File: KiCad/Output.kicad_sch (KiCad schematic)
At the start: 644 parts, among them J1 R_Phono_In, J10 VCC_IN, J11 VCC_OUT, J12 EMK_In, J15 Mic_Effekt_Out, J16 Mic_Effekt_Out, J17 Mic_Effekt_Out, J18 Mic_Effekt_Out, J19 Phono/Line_Out, J2 L_Phono_In, J20 Mic_Effekt_Out, J21 Conn_01x05_bridged, J22 EMK_In, J24 Mic_Effekt_In, J25 Mic_Effekt_In, J26 Phono/Line_In, J27 Mic_Effekt_In, J28 Pegel_Out, J29 Pegel_Out, J3 R_Line_In, J30 Pegel_In, J31 Pegel_In, J32 Pegel_In, J33 Pegel_In, J34 LED_Out, J35 LED_In, J36 VU_Meter_Out, J37 AUX_Send_3, J38 AUX_Send_1, J39 AUX_Send_2, J4 L_Line_In, J40 Bass_Out, J41 Kick_Out, J42 Mid_Out, J43 High_Out, J44 Line_Out_L, J45 Line_Out_R, J5 Mic_In, J6 Effekt_In, J7 AUX_RET_1, J8 AUX_RET_2, J9 AUX_RET_3, SW1 SW_DPST, SW10 SW_SPDT, SW11 SW_SPDT, SW12 SW_SPDT, SW2 SW_SPDT, SW3 SW_SPDT, SW4 SW_SPDT, SW5 SW_SPDT, SW6 SW_SPDT, SW7 SW_SPDT, SW8 SW_SPDT, SW9 SW_Rotary_1x4, U1 TL074, U10 TL074, U11 TL074, U12 TL074, U13 TL074, U14 TL074, U15 TL074, U16 TL074, U17 TL074, U18 TL074, U19 TL074, U2 TL074, U20 TL074, U21 TL074, U22 TL074, U23 TL074, U24 TL074, U25 INA128U, U3 TL074, U4 TL074, U5 TL074, U6 REC10K-2409, U7 REC10K-2415, U8 TL074, U9 TL074

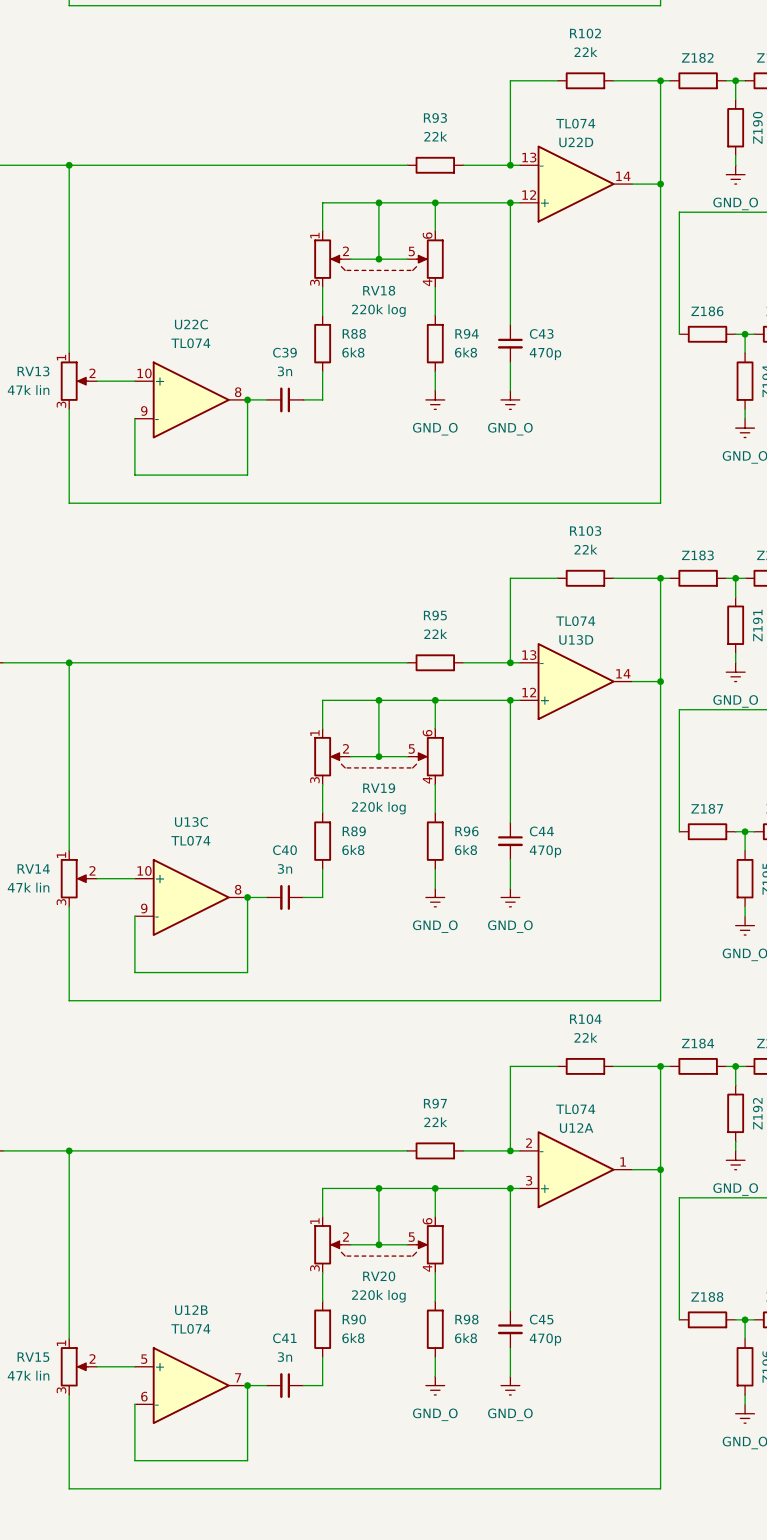
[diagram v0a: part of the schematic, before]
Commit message: PCB Update
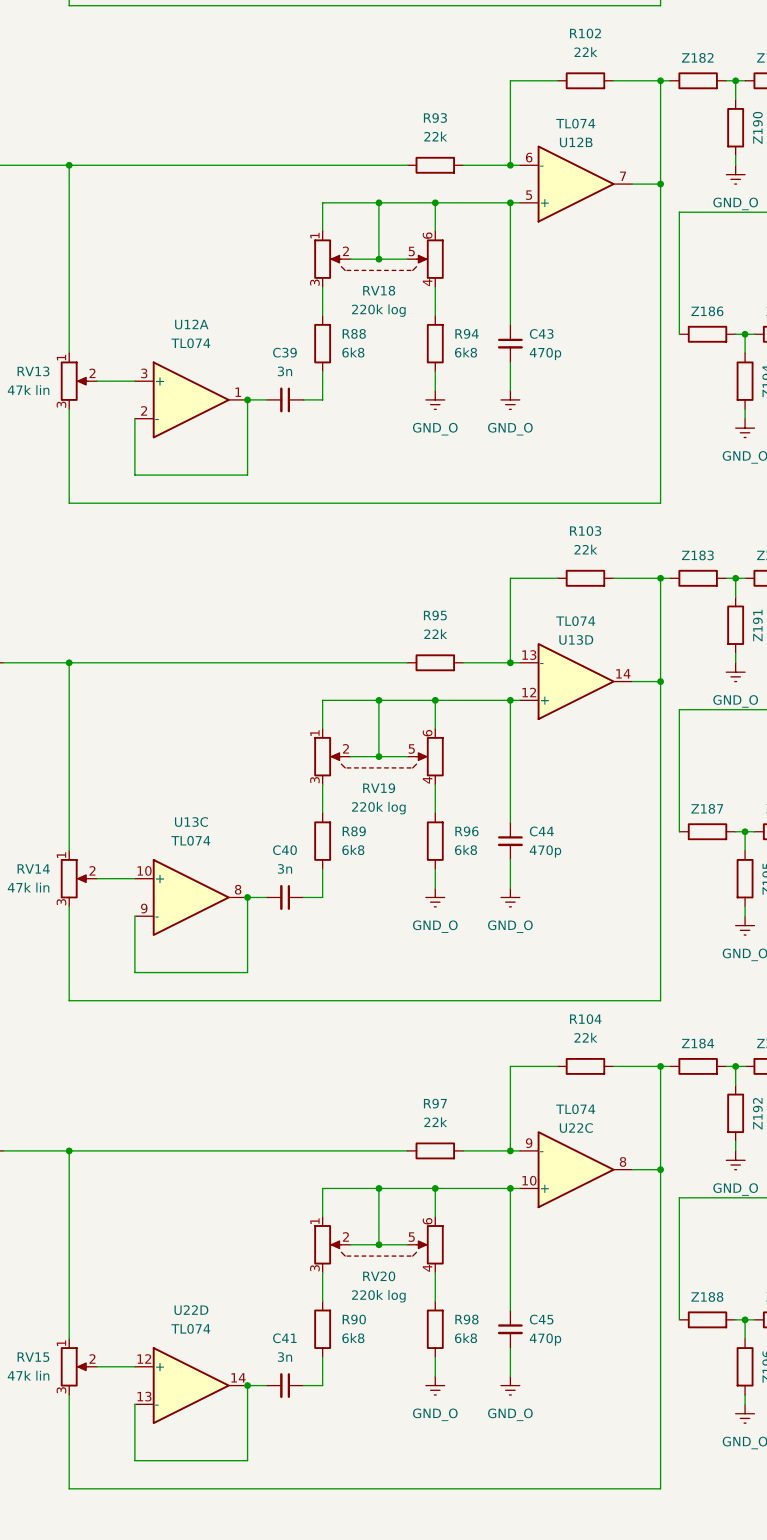
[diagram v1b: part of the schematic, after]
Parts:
- renumbered U22 to U12, U12 to U22
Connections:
- net at C45.1, RV20.1, RV20.2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: now also U22.10 (+); no longer U22.3 (+)
- net at C43.1, RV18.1, RV18.2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: now also U12.5 (+); no longer U12.12 (+)
- net at R102.1, R93.2: now also U12.6 (-); no longer U12.13 (-)
- net at R102.2, RV13.3, Z182.1: now also U12.7; no longer U12.14
- net at RV15.2: now also U22.12 (+); no longer U22.5 (+)
- net at R104.2, RV15.3, Z184.1: now also U22.8; no longer U22.1
- net at R104.1, R97.2: now also U22.9 (-); no longer U22.2 (-)
- net at RV13.2: now also U12.3 (+); no longer U12.10 (+)
- new net: C41.2, U22.13 (-), U22.14
- new net: C39.2, U12.1, U12.2 (-)
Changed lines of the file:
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@@
 		(at 613.41 140.97 0)
 		(mirror x)
-		(unit 4)
+		(unit 2)
 		(exclude_from_sim no)
 		(in_bom yes)
 		(on_board yes)
 		(dnp no)
-		(property "Reference" "U22"
+		(property "Reference" "U12"
 			(at 613.41 135.382 0)
 			(effects
@@
 			(project "DiKo_PreAmp"
 				(path "/81a92cd6-862a-4567-ad33-f8a3bc120591"
-					(reference "U22")
-					(unit 4)
+					(reference "U12")
+					(unit 2)
 				)
 			)
@@
 		(lib_id "Amplifier_Operational:TL074")
 		(at 561.34 170.18 0)
-		(unit 3)
+		(unit 1)
 		(exclude_from_sim no)
 		(in_bom yes)
@@
 		(dnp no)
 		(fields_autoplaced yes)
-		(property "Reference" "U22"
+		(property "Reference" "U12"
 			(at 561.34 160.02 0)
 			(effects
@@
 			(project "DiKo_PreAmp"
 				(path "/81a92cd6-862a-4567-ad33-f8a3bc120591"
-					(reference "U22")
-					(unit 3)
+					(reference "U12")
+					(unit 1)
 				)
 			)
@@
 		(at 613.41 274.32 0)
 		(mirror x)
-		(unit 1)
+		(unit 3)
 		(exclude_from_sim no)
 		(in_bom yes)
 		(on_board yes)
 		(dnp no)
-		(property "Reference" "U12"
+		(property "Reference" "U22"
 			(at 613.41 268.732 0)
 			(effects
@@
 			(project "DiKo_PreAmp"
 				(path "/81a92cd6-862a-4567-ad33-f8a3bc120591"
-					(reference "U12")
-					(unit 1)
+					(reference "U22")
+					(unit 3)
 				)
 			)
@@
 		(lib_id "Amplifier_Operational:TL074")
 		(at 561.34 303.53 0)
-		(unit 2)
+		(unit 4)
 		(exclude_from_sim no)
 		(in_bom yes)
@@
 		(dnp no)
 		(fields_autoplaced yes)
-		(property "Reference" "U12"
+		(property "Reference" "U22"
 			(at 561.34 293.37 0)
 			(effects
@@
 			(project "DiKo_PreAmp"
 				(path "/81a92cd6-862a-4567-ad33-f8a3bc120591"
-					(reference "U12")
-					(unit 2)
+					(reference "U22")
+					(unit 4)
 				)
 			)
